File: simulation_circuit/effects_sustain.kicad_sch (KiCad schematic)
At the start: 16 parts, among them Q1 BC547

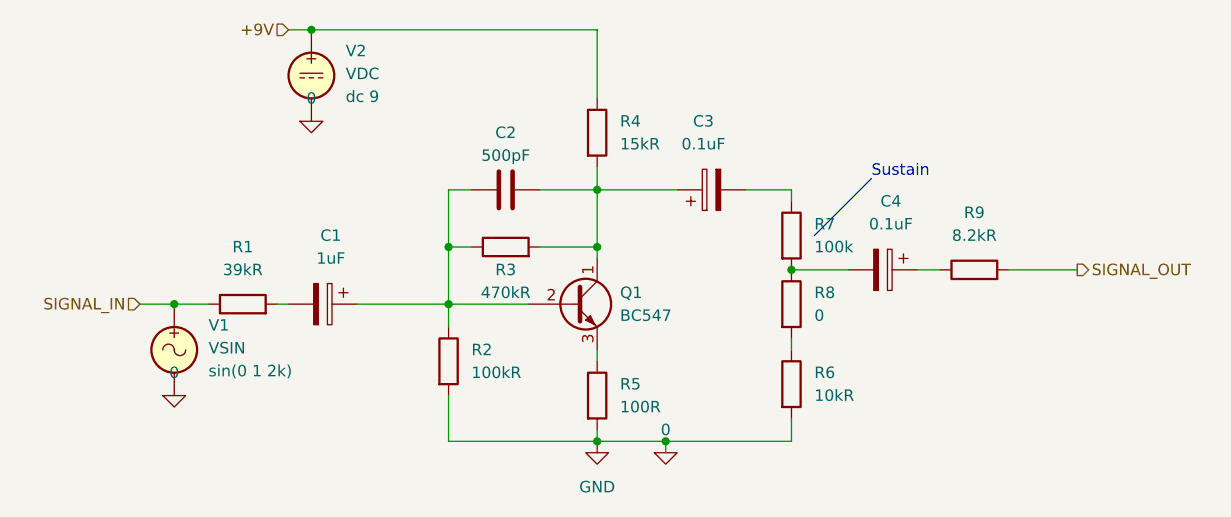
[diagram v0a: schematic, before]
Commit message: WIP
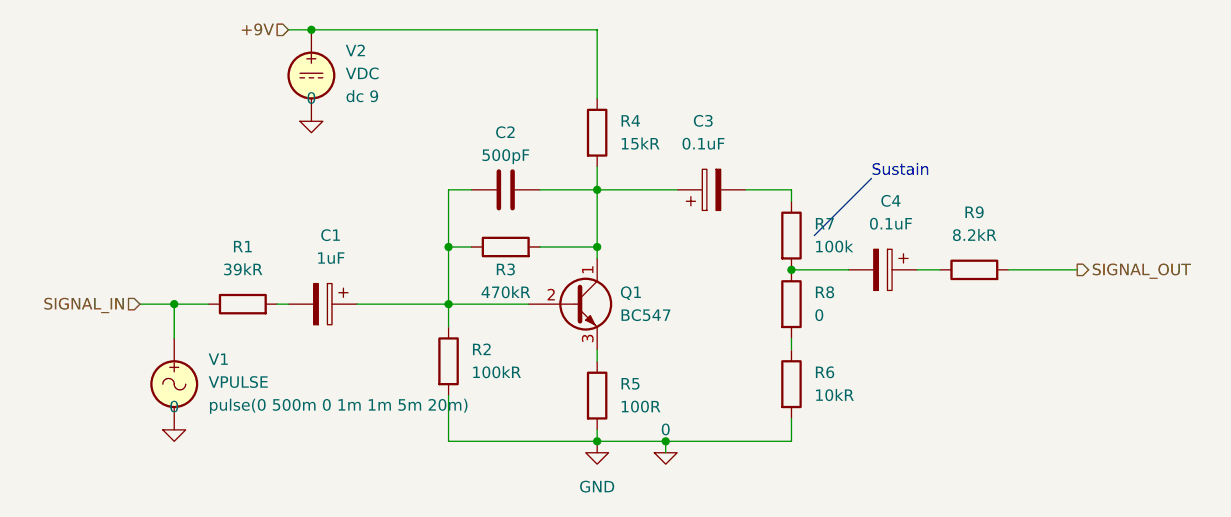
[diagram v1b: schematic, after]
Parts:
- V1: value VSIN -> VPULSE; Spice_Model sin(0 1 2k) -> pulse(0 500m 0 1m 1m 5m 20m)
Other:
- moved on the sheet: V1
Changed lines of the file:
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@@
   (junction (at 116.84 63.5) (diameter 0) (color 0 0 0 0)
   )
+  (junction (at 148.59 109.22) (diameter 0) (color 0 0 0 0)
+  )
+  (junction (at 148.59 81.28) (diameter 0) (color 0 0 0 0)
+  )
+  (junction (at 132.08 93.98) (diameter 0) (color 0 0 0 0)
+  )
+  (junction (at 148.59 87.63) (diameter 0) (color 0 0 0 0)
+  )
+  (junction (at 132.08 87.63) (diameter 0) (color 0 0 0 0)
+  )
   (junction (at 101.6 93.98) (diameter 0) (color 0 0 0 0)
   )
-  (junction (at 148.59 109.22) (diameter 0) (color 0 0 0 0)
-  )
-  (junction (at 148.59 81.28) (diameter 0) (color 0 0 0 0)
-  )
-  (junction (at 132.08 93.98) (diameter 0) (color 0 0 0 0)
-  )
-  (junction (at 148.59 87.63) (diameter 0) (color 0 0 0 0)
-  )
-  (junction (at 132.08 87.63) (diameter 0) (color 0 0 0 0)
-  )
   (junction (at 156.21 109.22) (diameter 0) (color 0 0 0 0)
   )
@@
   )
   (wire (pts (xy 170.18 81.28) (xy 170.18 82.55))
+    (stroke (width 0) (type default) (color 0 0 0 0))
+  )
+  (wire (pts (xy 101.6 93.98) (xy 101.6 97.79))
     (stroke (width 0) (type default) (color 0 0 0 0))
   )
@@
     (pin "2")
   )
-  (symbol (lib_id "pspice:0") (at 101.6 104.14 0) (unit 1)
-    (in_bom yes) (on_board yes) (fields_autoplaced)
-    (property "Reference" "#GND01" (id 0) (at 101.6 106.68 0)
-      (effects (font (size 1.27 1.27)) hide)
-    )
-    (property "Value" "0" (id 1) (at 101.6 101.6 0))
-    (property "Footprint" "" (id 2) (at 101.6 104.14 0)
-      (effects (font (size 1.27 1.27)) hide)
-    )
-    (property "Datasheet" "~" (id 3) (at 101.6 104.14 0)
+  (symbol (lib_id "pspice:0") (at 101.6 107.95 0) (unit 1)
+    (in_bom yes) (on_board yes) (fields_autoplaced)
+    (property "Reference" "#GND01" (id 0) (at 101.6 110.49 0)
+      (effects (font (size 1.27 1.27)) hide)
+    )
+    (property "Value" "0" (id 1) (at 101.6 105.41 0))
+    (property "Footprint" "" (id 2) (at 101.6 107.95 0)
+      (effects (font (size 1.27 1.27)) hide)
+    )
+    (property "Datasheet" "~" (id 3) (at 101.6 107.95 0)
       (effects (font (size 1.27 1.27)) hide)
     )
@@
     (pin "2")
   )
-  (symbol (lib_id "Simulation_SPICE:VSIN") (at 101.6 99.06 0) (unit 1)
-    (in_bom yes) (on_board yes) (fields_autoplaced)
-    (property "Reference" "V1" (id 0) (at 105.41 96.3301 0)
-      (effects (font (size 1.27 1.27)) (justify left))
-    )
-    (property "Value" "VSIN" (id 1) (at 105.41 98.8701 0)
-      (effects (font (size 1.27 1.27)) (justify left))
-    )
-    (property "Footprint" "" (id 2) (at 101.6 99.06 0)
-      (effects (font (size 1.27 1.27)) hide)
-    )
-    (property "Datasheet" "~" (id 3) (at 101.6 99.06 0)
-      (effects (font (size 1.27 1.27)) hide)
-    )
-    (property "Spice_Netlist_Enabled" "Y" (id 4) (at 101.6 99.06 0)
+  (symbol (lib_id "Simulation_SPICE:VSIN") (at 101.6 102.87 0) (unit 1)
+    (in_bom yes) (on_board yes) (fields_autoplaced)
+    (property "Reference" "V1" (id 0) (at 105.41 100.1401 0)
+      (effects (font (size 1.27 1.27)) (justify left))
+    )
+    (property "Value" "VPULSE" (id 1) (at 105.41 102.6801 0)
+      (effects (font (size 1.27 1.27)) (justify left))
+    )
+    (property "Footprint" "" (id 2) (at 101.6 102.87 0)
+      (effects (font (size 1.27 1.27)) hide)
+    )
+    (property "Datasheet" "~" (id 3) (at 101.6 102.87 0)
+      (effects (font (size 1.27 1.27)) hide)
+    )
+    (property "Spice_Netlist_Enabled" "Y" (id 4) (at 101.6 102.87 0)
       (effects (font (size 1.27 1.27)) (justify left) hide)
     )
-    (property "Spice_Primitive" "V" (id 5) (at 101.6 99.06 0)
+    (property "Spice_Primitive" "V" (id 5) (at 101.6 102.87 0)
       (effects (font (size 1.27 1.27)) (justify left) hide)
     )
-    (property "Spice_Model" "sin(0 1 2k)" (id 6) (at 105.41 101.4101 0)
-      (effects (font (size 1.27 1.27)) (justify left))
-    )
+    (property "Spice_Model" "pulse(0 500m 0 1m 1m 5m 20m)" (id 6) (at 105.41 105.2201 0)
+      (effects (font (size 1.27 1.27)) (justify left))
+    )
